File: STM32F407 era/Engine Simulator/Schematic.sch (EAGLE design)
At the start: 25 parts, among them U1 MAX13052ESA+, U2 AD5293BRUZ-100, U3 AD5024BRUZ, X4 057-006-1

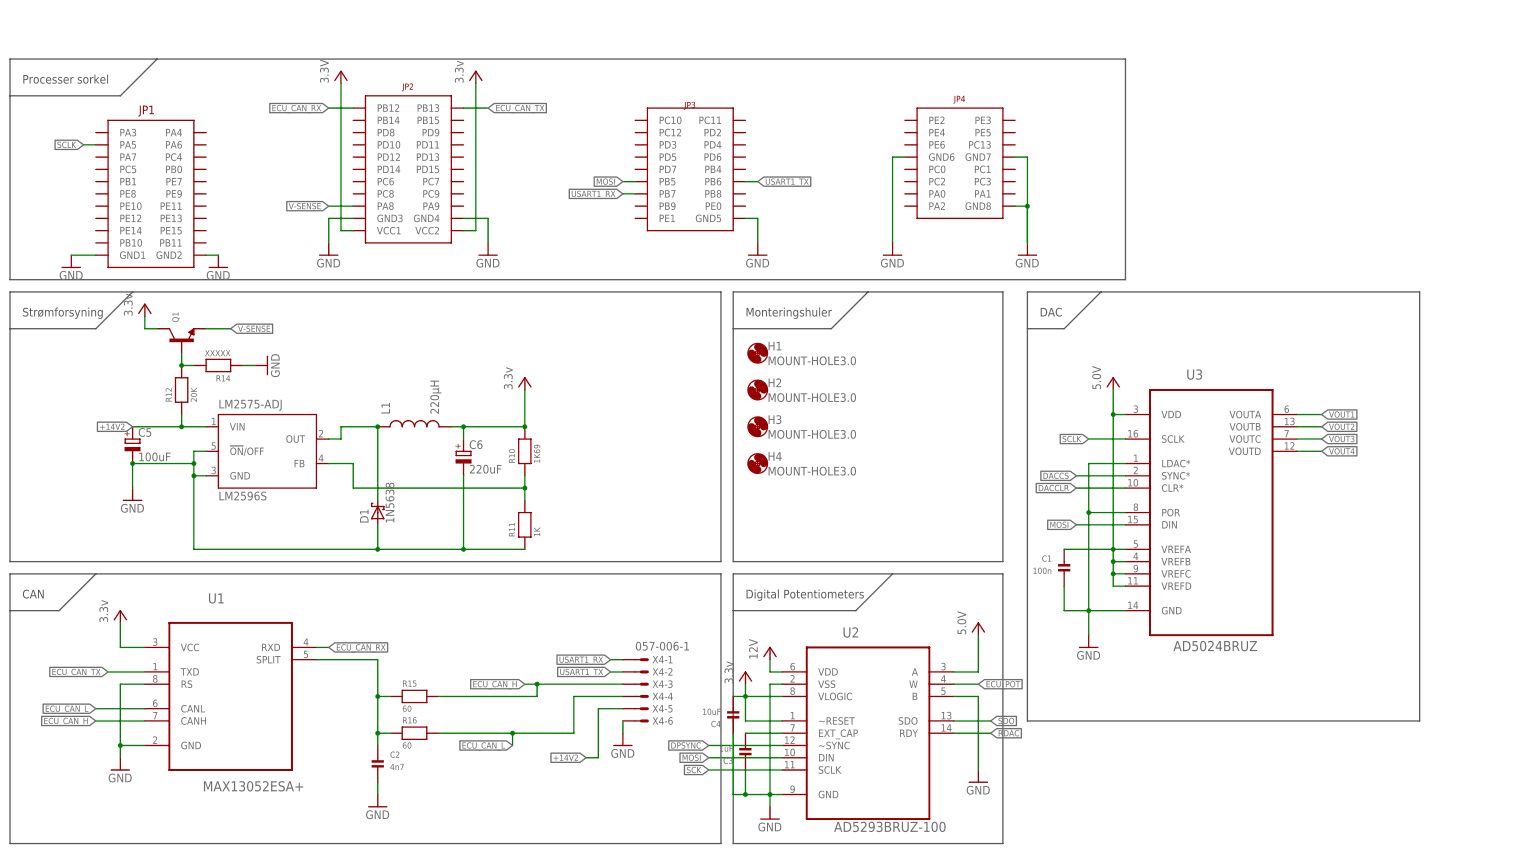
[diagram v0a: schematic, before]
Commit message: no message
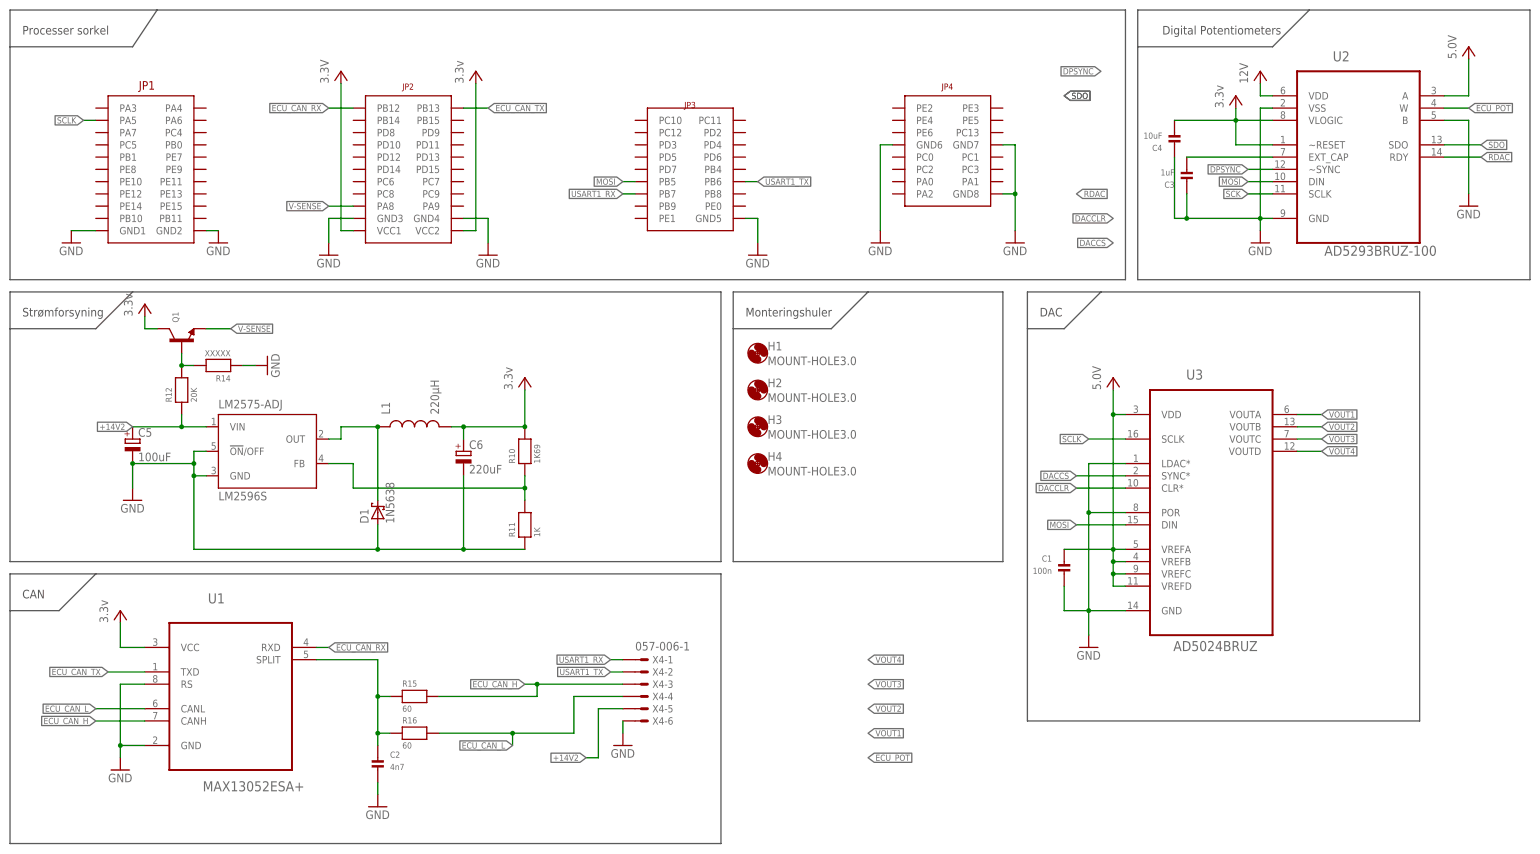
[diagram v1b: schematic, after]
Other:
- moved on the sheet: C3, C4, U2
